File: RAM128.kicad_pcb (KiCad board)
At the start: 4 copper layers, 71.6 x 35.7 mm, 69 parts, among them J1 AppleIIBus, U1 621024, U10 742G04GW, U11 74LVC1G125GW, U12 74LVC1G08GW, U13 74LVC1G32GW, U14 74LVC1G08GW, U15 742G04GW, U16 74LVC1G32GW, U17 742G04GW, U18 742G04GW, U19 74LVC1G08GW, U2 74AHC245PW, U20 742G04GW, U21 74LVC1G32GW, U22 74LVC1G08GW, U23 74LVC1G08GW, U24 74LVC1G08GW, U25 742G04GW, U26 74LVC1G08GW, U27 74LVC1G08GW, U28 74LVC1G08GW, U29 742G04GW, U3 74HCT273PW, U30 74LVC1G08GW, U31 742G04GW, U32 74LVC1G32GW, U33 742G04GW, U34 74LVC1G32GW, U35 XC6206PxxxMR, U4 74HCT273PW, U5 74LVC1G08GW, U6 74LVC1G32GW, U7 74LVC1G08GW, U8 74LVC1G32GW, U9 74LVC1G08GW

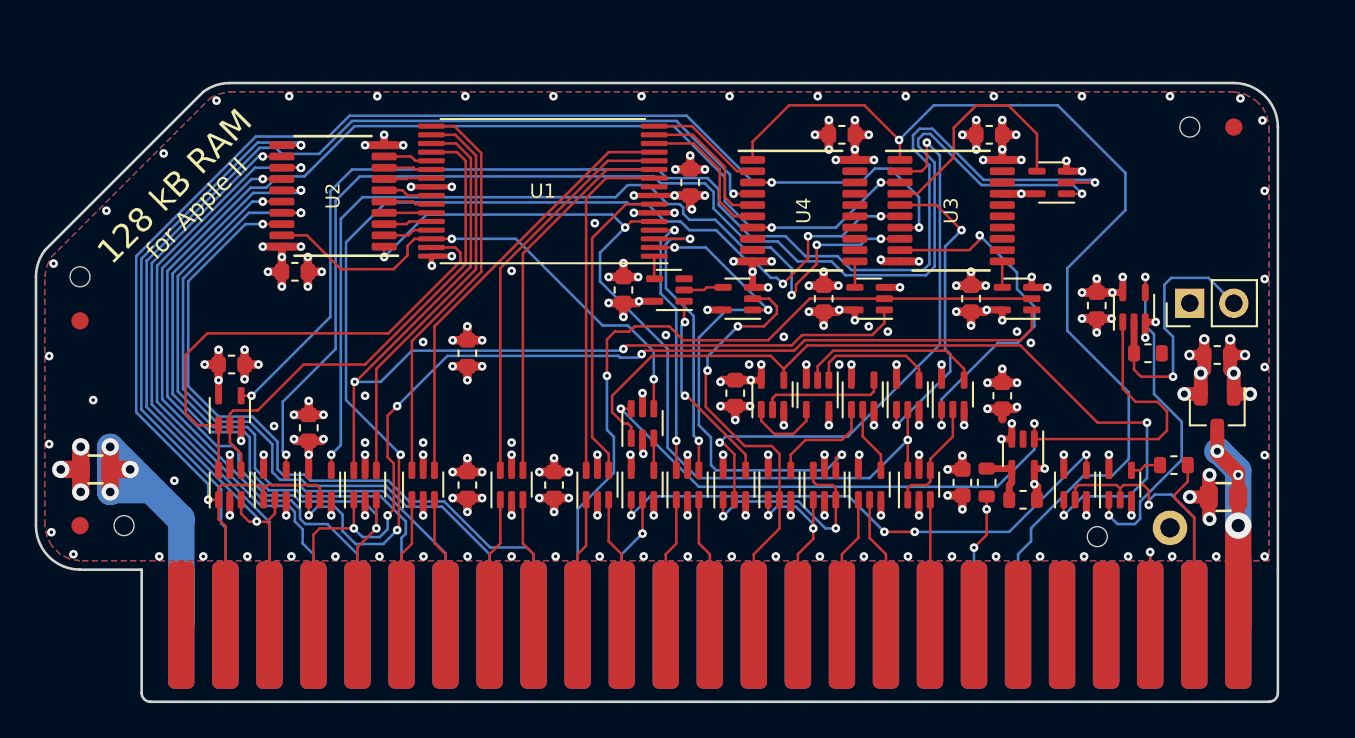
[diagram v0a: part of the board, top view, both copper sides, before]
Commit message: little logic done
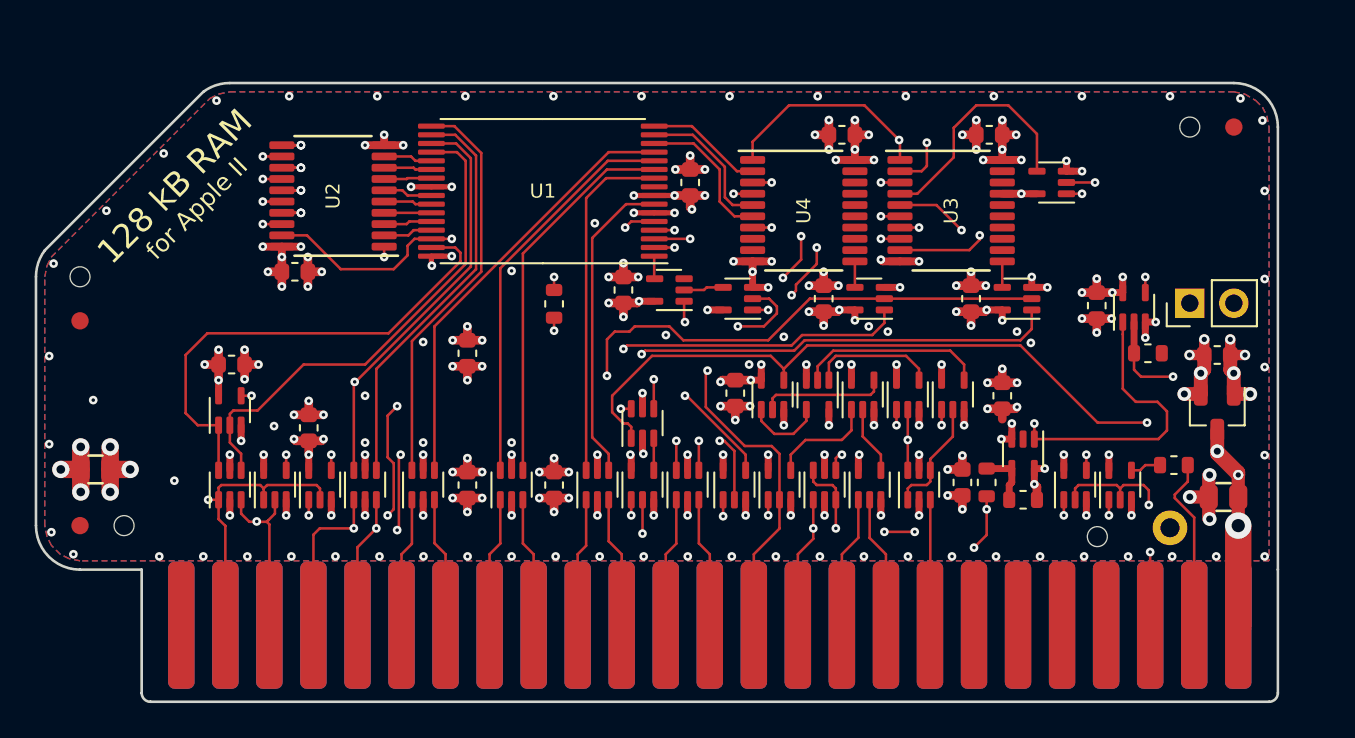
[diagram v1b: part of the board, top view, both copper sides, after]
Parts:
- removed the C2 at (92.7, 119.6)
- removed the C2 at (79.1, 120.2)
- removed the C2 at (122.8, 107.0)
- removed the C2 at (105.5, 109.8)
- removed the C2 at (82.8, 114.9)
- removed the C2 at (121.2, 127.0)
- removed the C8 at (83.5, 123.9)
- added C13: 2u2, stdpads:C_0603, F.Cu at (122.8, 107.0)
- added C15: 2u2, stdpads:C_0603, F.Cu at (105.5, 109.8)
- added C16: 2u2, stdpads:C_0603, F.Cu at (82.8, 114.9)
- added C17: 2u2, stdpads:C_0603, F.Cu at (121.2, 127.0)
- added C19: 2u2, stdpads:C_0603, F.Cu at (83.5, 123.9)
- added C5: 2u2, stdpads:C_0603, F.Cu at (79.1, 120.2)
- added C9: 2u2, stdpads:C_0603, F.Cu at (92.7, 119.6)
- added R2: 33, stdpads:R_0603, F.Cu at (97.7, 116.8)
- R3, R4: value 30 -> 33
- U1: value 621024 -> LY62W1024
- U10, U15, U17, U18, U20, U25, U29, U31, U33: value 742G04GW -> 74LVC2G04GW
- renumbered C2 to C1, C8 to C10, C2 to C14, C8 to C18, C8 to C4, C8 to C6
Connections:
- U31 pad 4: /R~CS~ -> Net-(R2-Pad2)
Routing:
- net Net-(R2-Pad2): track 0.00 -> 10.5 mm, vias 0 -> 2
- net /R~CS~: track 29.3 -> 19.2 mm
- net GND: vias 170 -> 169
- net +3V3: vias 87 -> 88
- added copper zone on B.Cu, net +3V3
- added copper zone on In2.Cu, net GND
- removed copper zone on In2.Cu, net +3V3
- removed copper zone on B.Cu, net GND

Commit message: Revert "little logic done"
This reverts commit c8f7fd6b2897fba301a82931860b3ed280e7265e.
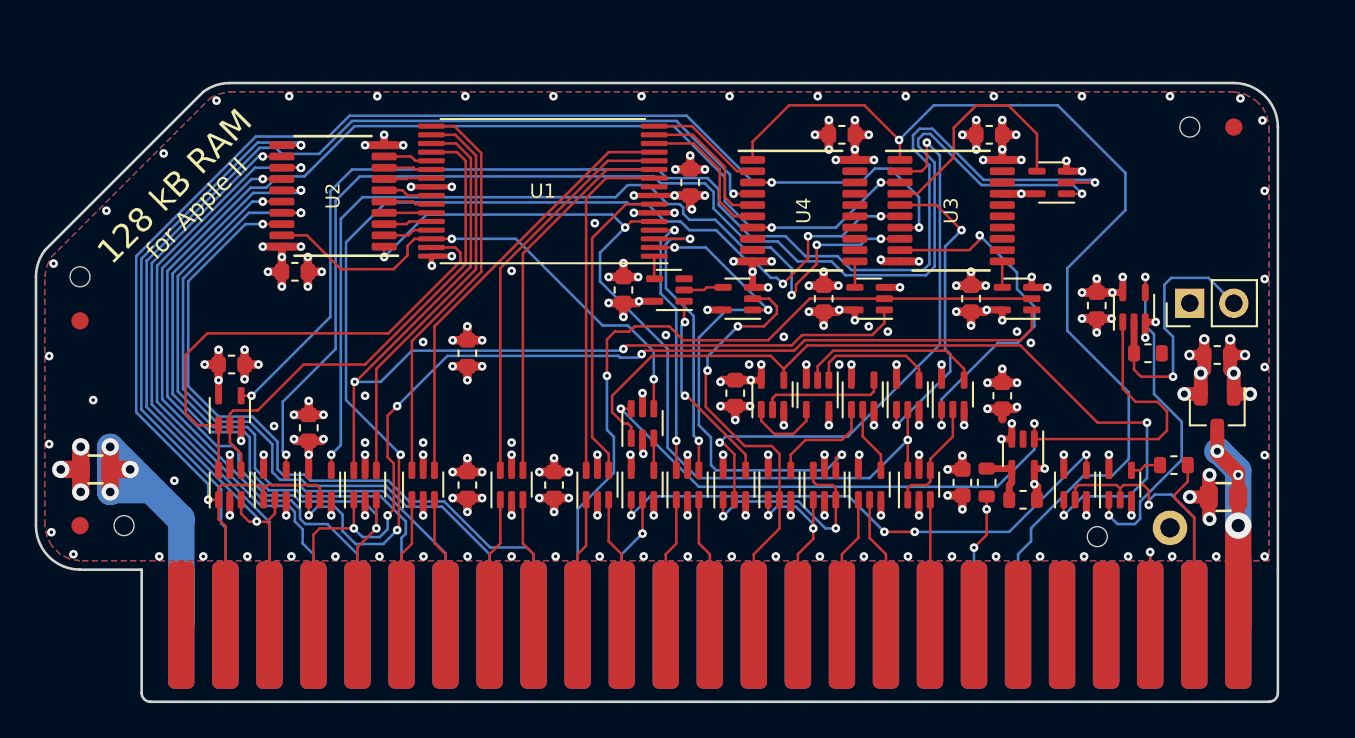
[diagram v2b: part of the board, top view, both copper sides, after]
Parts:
- removed C13, C15, C16, C17, C19, C5, C9: 2u2, stdpads:C_0603
- removed R2: 33, stdpads:R_0603
- added C2: 2u2, stdpads:C_0603, F.Cu at (92.7, 119.6)
- added C2: 2u2, stdpads:C_0603, F.Cu at (79.1, 120.2)
- added C2: 2u2, stdpads:C_0603, F.Cu at (122.8, 107.0)
- added C2: 2u2, stdpads:C_0603, F.Cu at (105.5, 109.8)
- added C2: 2u2, stdpads:C_0603, F.Cu at (82.8, 114.9)
- added C2: 2u2, stdpads:C_0603, F.Cu at (121.2, 127.0)
- added C8: 2u2, stdpads:C_0603, F.Cu at (83.5, 123.9)
- R3, R4: value 33 -> 30
- U1: value LY62W1024 -> 621024
- U10, U15, U17, U18, U20, U25, U29, U31, U33: value 74LVC2G04GW -> 742G04GW
- renumbered C14 to C2, C1 to C2, C6 to C8, C4 to C8, C10 to C8, C18 to C8
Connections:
- U31 pad 4: Net-(R2-Pad2) -> /R~CS~
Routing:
- net Net-(R2-Pad2): track 10.5 -> 0.00 mm, vias 2 -> 0
- net /R~CS~: track 19.2 -> 29.3 mm
- net GND: vias 169 -> 170
- net +3V3: vias 88 -> 87
- added copper zone on In2.Cu, net +3V3
- added copper zone on B.Cu, net GND
- removed copper zone on B.Cu, net +3V3
- removed copper zone on In2.Cu, net GND
